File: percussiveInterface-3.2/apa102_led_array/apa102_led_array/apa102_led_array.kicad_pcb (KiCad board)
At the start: 2 copper layers, 167 x 10.2 mm, 49 parts

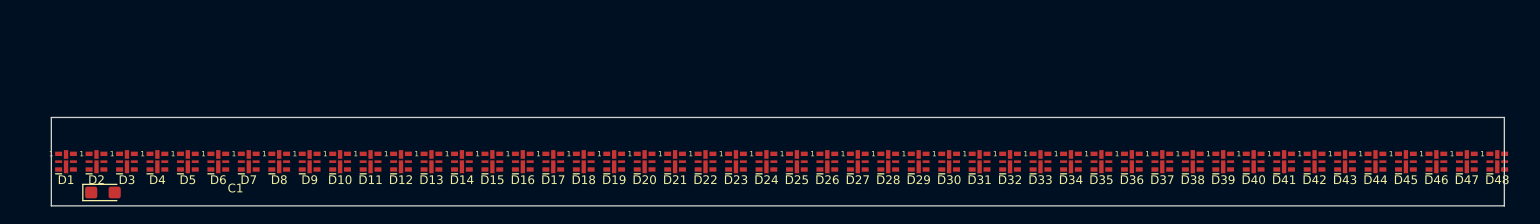
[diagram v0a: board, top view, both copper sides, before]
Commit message: many changes
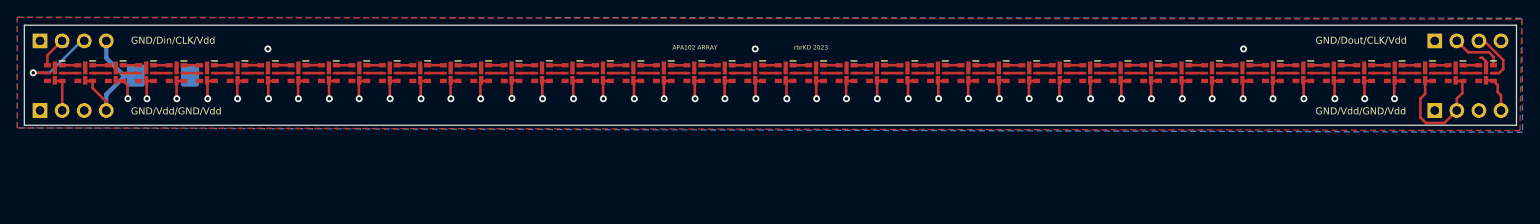
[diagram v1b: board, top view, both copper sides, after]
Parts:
- added REF**: PinHeader_1x04_P2.54mm_Vertical, Connector_PinHeader_2.54mm:PinHeader_1x04_P2.54mm_Vertical, B.Cu at (36.8, 29.3)
- added REF**: PinHeader_1x04_P2.54mm_Vertical, Connector_PinHeader_2.54mm:PinHeader_1x04_P2.54mm_Vertical, B.Cu at (197.1, 37.3)
- added REF**: PinHeader_1x04_P2.54mm_Vertical, Connector_PinHeader_2.54mm:PinHeader_1x04_P2.54mm_Vertical, B.Cu at (197.1, 29.3)
- added REF**: PinHeader_1x04_P2.54mm_Vertical, Connector_PinHeader_2.54mm:PinHeader_1x04_P2.54mm_Vertical, B.Cu at (36.8, 37.3)
- C1: footprint Capacitor_Tantalum_SMD:CP_EIA-3216-18_Kemet-A -> Capacitor_Tantalum_SMD:CP_EIA-7343-15_Kemet-W; moved to B.Cu
- moved C1 15.1 mm to (50.9, 33.3)
- moved D10 10.3 mm to (70.0, 33.0), turned to 180 degrees
- moved D11 10.3 mm to (73.5, 33.0), turned to 180 degrees
- moved D12 10.3 mm to (77.0, 33.0), turned to 180 degrees
- moved D13 10.3 mm to (80.5, 33.0), turned to 180 degrees
- moved D14 10.3 mm to (84.0, 33.0), turned to 180 degrees
- moved D15 10.3 mm to (87.5, 33.0), turned to 180 degrees
- moved D16 10.3 mm to (91.0, 33.0), turned to 180 degrees
- moved D17 10.3 mm to (94.5, 33.0), turned to 180 degrees
- moved D18 10.3 mm to (98.0, 33.0), turned to 180 degrees
- moved D19 10.3 mm to (101.5, 33.0), turned to 180 degrees
- moved D20 10.3 mm to (105.0, 33.0), turned to 180 degrees
- moved D21 10.3 mm to (108.5, 33.0), turned to 180 degrees
- moved D22 10.3 mm to (112.0, 33.0), turned to 180 degrees
- moved D23 10.3 mm to (115.5, 33.0), turned to 180 degrees
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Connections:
- D10 pad 2: Net-(D1-CKO) -> Net-(D10-CKO)
- D10 pad 3: Net-(D1-SDO) -> Net-(D10-SDO)
- D10 pad 4: DATA_IN -> Net-(D10-SDI)
- D10 pad 5: CLK_IN -> Net-(D10-CKI)
- D11 pad 2: Net-(D1-CKO) -> Net-(D11-CKO)
- D11 pad 3: Net-(D1-SDO) -> Net-(D11-SDO)
- D11 pad 4: DATA_IN -> Net-(D10-SDO)
- D11 pad 5: CLK_IN -> Net-(D10-CKO)
- D12 pad 2: Net-(D1-CKO) -> Net-(D12-CKO)
- D12 pad 3: Net-(D1-SDO) -> Net-(D12-SDO)
- D12 pad 4: DATA_IN -> Net-(D11-SDO)
- D12 pad 5: CLK_IN -> Net-(D11-CKO)
- D13 pad 2: Net-(D1-CKO) -> Net-(D13-CKO)
- D13 pad 3: Net-(D1-SDO) -> Net-(D13-SDO)
- D13 pad 4: DATA_IN -> Net-(D12-SDO)
- D13 pad 5: CLK_IN -> Net-(D12-CKO)
- D14 pad 2: Net-(D1-CKO) -> Net-(D14-CKO)
- D14 pad 3: Net-(D1-SDO) -> Net-(D14-SDO)
- D14 pad 4: DATA_IN -> Net-(D13-SDO)
- D14 pad 5: CLK_IN -> Net-(D13-CKO)
- D15 pad 2: Net-(D1-CKO) -> Net-(D15-CKO)
- D15 pad 3: Net-(D1-SDO) -> Net-(D15-SDO)
- D15 pad 4: DATA_IN -> Net-(D14-SDO)
- D15 pad 5: CLK_IN -> Net-(D14-CKO)
- D16 pad 2: Net-(D1-CKO) -> Net-(D16-CKO)
- D16 pad 3: Net-(D1-SDO) -> Net-(D16-SDO)
- D16 pad 4: DATA_IN -> Net-(D15-SDO)
- D16 pad 5: CLK_IN -> Net-(D15-CKO)
- D17 pad 2: Net-(D1-CKO) -> Net-(D17-CKO)
- D17 pad 3: Net-(D1-SDO) -> Net-(D17-SDO)
- D17 pad 4: DATA_IN -> Net-(D16-SDO)
- D17 pad 5: CLK_IN -> Net-(D16-CKO)
- D18 pad 2: Net-(D1-CKO) -> Net-(D18-CKO)
- D18 pad 3: Net-(D1-SDO) -> Net-(D18-SDO)
- D18 pad 4: DATA_IN -> Net-(D17-SDO)
- D18 pad 5: CLK_IN -> Net-(D17-CKO)
- D19 pad 2: Net-(D1-CKO) -> Net-(D19-CKO)
- D19 pad 3: Net-(D1-SDO) -> Net-(D19-SDO)
- D19 pad 4: DATA_IN -> Net-(D18-SDO)
- D19 pad 5: CLK_IN -> Net-(D18-CKO)
- D2 pad 2: Net-(D1-CKO) -> Net-(D2-CKO)
- D2 pad 3: Net-(D1-SDO) -> Net-(D2-SDO)
- D2 pad 4: DATA_IN -> Net-(D1-SDO)
- D2 pad 5: CLK_IN -> Net-(D1-CKO)
- D20 pad 2: Net-(D1-CKO) -> Net-(D20-CKO)
- D20 pad 3: Net-(D1-SDO) -> Net-(D20-SDO)
- D20 pad 4: DATA_IN -> Net-(D19-SDO)
- D20 pad 5: CLK_IN -> Net-(D19-CKO)
- D21 pad 2: Net-(D1-CKO) -> Net-(D21-CKO)
- D21 pad 3: Net-(D1-SDO) -> Net-(D21-SDO)
- D21 pad 4: DATA_IN -> Net-(D20-SDO)
- D21 pad 5: CLK_IN -> Net-(D20-CKO)
- D22 pad 2: Net-(D1-CKO) -> Net-(D22-CKO)
- D22 pad 3: Net-(D1-SDO) -> Net-(D22-SDO)
- D22 pad 4: DATA_IN -> Net-(D21-SDO)
- D22 pad 5: CLK_IN -> Net-(D21-CKO)
- D23 pad 2: Net-(D1-CKO) -> Net-(D23-CKO)
- D23 pad 3: Net-(D1-SDO) -> Net-(D23-SDO)
- D23 pad 4: DATA_IN -> Net-(D22-SDO)
- D23 pad 5: CLK_IN -> Net-(D22-CKO)
- D24 pad 2: Net-(D1-CKO) -> Net-(D24-CKO)
- D24 pad 3: Net-(D1-SDO) -> Net-(D24-SDO)
- D24 pad 4: DATA_IN -> Net-(D23-SDO)
- D24 pad 5: CLK_IN -> Net-(D23-CKO)
- D25 pad 2: Net-(D1-CKO) -> Net-(D25-CKO)
- D25 pad 3: Net-(D1-SDO) -> Net-(D25-SDO)
- D25 pad 4: DATA_IN -> Net-(D24-SDO)
- D25 pad 5: CLK_IN -> Net-(D24-CKO)
- D26 pad 2: Net-(D1-CKO) -> Net-(D26-CKO)
- D26 pad 3: Net-(D1-SDO) -> Net-(D26-SDO)
- D26 pad 4: DATA_IN -> Net-(D25-SDO)
- D26 pad 5: CLK_IN -> Net-(D25-CKO)
- D27 pad 2: Net-(D1-CKO) -> Net-(D27-CKO)
- D27 pad 3: Net-(D1-SDO) -> Net-(D27-SDO)
- D27 pad 4: DATA_IN -> Net-(D26-SDO)
- D27 pad 5: CLK_IN -> Net-(D26-CKO)
- D28 pad 2: Net-(D1-CKO) -> Net-(D28-CKO)
- D28 pad 3: Net-(D1-SDO) -> Net-(D28-SDO)
- D28 pad 4: DATA_IN -> Net-(D27-SDO)
- D28 pad 5: CLK_IN -> Net-(D27-CKO)
- D29 pad 2: Net-(D1-CKO) -> Net-(D29-CKO)
- D29 pad 3: Net-(D1-SDO) -> Net-(D29-SDO)
- D29 pad 4: DATA_IN -> Net-(D28-SDO)
- D29 pad 5: CLK_IN -> Net-(D28-CKO)
- D3 pad 2: Net-(D1-CKO) -> Net-(D3-CKO)
- D3 pad 3: Net-(D1-SDO) -> Net-(D3-SDO)
- D3 pad 4: DATA_IN -> Net-(D2-SDO)
- D3 pad 5: CLK_IN -> Net-(D2-CKO)
- D30 pad 2: Net-(D1-CKO) -> Net-(D30-CKO)
- D30 pad 3: Net-(D1-SDO) -> Net-(D30-SDO)
- D30 pad 4: DATA_IN -> Net-(D29-SDO)
- D30 pad 5: CLK_IN -> Net-(D29-CKO)
- D31 pad 2: Net-(D1-CKO) -> Net-(D31-CKO)
- D31 pad 3: Net-(D1-SDO) -> Net-(D31-SDO)
- D31 pad 4: DATA_IN -> Net-(D30-SDO)
- D31 pad 5: CLK_IN -> Net-(D30-CKO)
- D32 pad 2: Net-(D1-CKO) -> Net-(D32-CKO)
- D32 pad 3: Net-(D1-SDO) -> Net-(D32-SDO)
- D32 pad 4: DATA_IN -> Net-(D31-SDO)
- D32 pad 5: CLK_IN -> Net-(D31-CKO)
- D33 pad 2: Net-(D1-CKO) -> Net-(D33-CKO)
- D33 pad 3: Net-(D1-SDO) -> Net-(D33-SDO)
- D33 pad 4: DATA_IN -> Net-(D32-SDO)
- D33 pad 5: CLK_IN -> Net-(D32-CKO)
- D34 pad 2: Net-(D1-CKO) -> Net-(D34-CKO)
- D34 pad 3: Net-(D1-SDO) -> Net-(D34-SDO)
- D34 pad 4: DATA_IN -> Net-(D33-SDO)
- D34 pad 5: CLK_IN -> Net-(D33-CKO)
- D35 pad 2: Net-(D1-CKO) -> Net-(D35-CKO)
- D35 pad 3: Net-(D1-SDO) -> Net-(D35-SDO)
- D35 pad 4: DATA_IN -> Net-(D34-SDO)
- D35 pad 5: CLK_IN -> Net-(D34-CKO)
- D36 pad 2: Net-(D1-CKO) -> Net-(D36-CKO)
- D36 pad 3: Net-(D1-SDO) -> Net-(D36-SDO)
- D36 pad 4: DATA_IN -> Net-(D35-SDO)
- D36 pad 5: CLK_IN -> Net-(D35-CKO)
- D37 pad 2: Net-(D1-CKO) -> Net-(D37-CKO)
- D37 pad 3: Net-(D1-SDO) -> Net-(D37-SDO)
- D37 pad 4: DATA_IN -> Net-(D36-SDO)
- D37 pad 5: CLK_IN -> Net-(D36-CKO)
- D38 pad 2: Net-(D1-CKO) -> Net-(D38-CKO)
- D38 pad 3: Net-(D1-SDO) -> Net-(D38-SDO)
- D38 pad 4: DATA_IN -> Net-(D37-SDO)
- D38 pad 5: CLK_IN -> Net-(D37-CKO)
- D39 pad 2: Net-(D1-CKO) -> Net-(D39-CKO)
- D39 pad 3: Net-(D1-SDO) -> Net-(D39-SDO)
- D39 pad 4: DATA_IN -> Net-(D38-SDO)
- D39 pad 5: CLK_IN -> Net-(D38-CKO)
- D4 pad 2: Net-(D1-CKO) -> Net-(D4-CKO)
- D4 pad 3: Net-(D1-SDO) -> Net-(D4-SDO)
- D4 pad 4: DATA_IN -> Net-(D3-SDO)
- D4 pad 5: CLK_IN -> Net-(D3-CKO)
- D40 pad 2: Net-(D1-CKO) -> Net-(D40-CKO)
- D40 pad 3: Net-(D1-SDO) -> Net-(D40-SDO)
- D40 pad 4: DATA_IN -> Net-(D39-SDO)
- D40 pad 5: CLK_IN -> Net-(D39-CKO)
- D41 pad 2: Net-(D1-CKO) -> Net-(D41-CKO)
- D41 pad 3: Net-(D1-SDO) -> Net-(D41-SDO)
- D41 pad 4: DATA_IN -> Net-(D40-SDO)
- D41 pad 5: CLK_IN -> Net-(D40-CKO)
- D42 pad 2: Net-(D1-CKO) -> Net-(D42-CKO)
- D42 pad 3: Net-(D1-SDO) -> Net-(D42-SDO)
- D42 pad 4: DATA_IN -> Net-(D41-SDO)
- D42 pad 5: CLK_IN -> Net-(D41-CKO)
- D43 pad 2: Net-(D1-CKO) -> Net-(D43-CKO)
- D43 pad 3: Net-(D1-SDO) -> Net-(D43-SDO)
- D43 pad 4: DATA_IN -> Net-(D42-SDO)
- D43 pad 5: CLK_IN -> Net-(D42-CKO)
- D44 pad 2: Net-(D1-CKO) -> Net-(D44-CKO)
- D44 pad 3: Net-(D1-SDO) -> Net-(D44-SDO)
- D44 pad 4: DATA_IN -> Net-(D43-SDO)
- D44 pad 5: CLK_IN -> Net-(D43-CKO)
- D45 pad 2: Net-(D1-CKO) -> Net-(D45-CKO)
- D45 pad 3: Net-(D1-SDO) -> Net-(D45-SDO)
- D45 pad 4: DATA_IN -> Net-(D44-SDO)
- D45 pad 5: CLK_IN -> Net-(D44-CKO)
- D46 pad 2: Net-(D1-CKO) -> Net-(D46-CKO)
- D46 pad 3: Net-(D1-SDO) -> Net-(D46-SDO)
- D46 pad 4: DATA_IN -> Net-(D45-SDO)
- D46 pad 5: CLK_IN -> Net-(D45-CKO)
- D47 pad 2: Net-(D1-CKO) -> Net-(D47-CKO)
- D47 pad 3: Net-(D1-SDO) -> Net-(D47-SDO)
- D47 pad 4: DATA_IN -> Net-(D46-SDO)
- D47 pad 5: CLK_IN -> Net-(D46-CKO)
- D48 pad 2: Net-(D1-CKO) -> CLK_IN
- D48 pad 3: Net-(D1-SDO) -> DATA_IN
- D48 pad 4: DATA_IN -> Net-(D47-SDO)
- D48 pad 5: CLK_IN -> Net-(D47-CKO)
- D5 pad 2: Net-(D1-CKO) -> Net-(D5-CKO)
- D5 pad 3: Net-(D1-SDO) -> Net-(D5-SDO)
- D5 pad 4: DATA_IN -> Net-(D4-SDO)
- D5 pad 5: CLK_IN -> Net-(D4-CKO)
- D6 pad 2: Net-(D1-CKO) -> Net-(D6-CKO)
- D6 pad 3: Net-(D1-SDO) -> Net-(D6-SDO)
- D6 pad 4: DATA_IN -> Net-(D5-SDO)
- D6 pad 5: CLK_IN -> Net-(D5-CKO)
- D7 pad 2: Net-(D1-CKO) -> Net-(D7-CKO)
- D7 pad 3: Net-(D1-SDO) -> Net-(D7-SDO)
- D7 pad 4: DATA_IN -> Net-(D6-SDO)
- D7 pad 5: CLK_IN -> Net-(D6-CKO)
- D8 pad 2: Net-(D1-CKO) -> Net-(D8-CKO)
- D8 pad 3: Net-(D1-SDO) -> Net-(D8-SDO)
- D8 pad 4: DATA_IN -> Net-(D7-SDO)
- D8 pad 5: CLK_IN -> Net-(D7-CKO)
- D9 pad 2: Net-(D1-CKO) -> Net-(D10-CKI)
- D9 pad 3: Net-(D1-SDO) -> Net-(D10-SDI)
- D9 pad 4: DATA_IN -> Net-(D8-SDO)
- D9 pad 5: CLK_IN -> Net-(D8-CKO)
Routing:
- net Vdd: track 0.00 -> 164.0 mm, vias 0 -> 43
- net CLK_IN: track 0.00 -> 15.1 mm, vias 0 -> 1
- net DATA_IN: track 0.00 -> 10.1 mm
- net Net-(D47-SDO): track 0.00 -> 1.80 mm
- net Net-(D47-CKO): track 0.00 -> 1.80 mm
- net Net-(D46-SDO): track 0.00 -> 1.80 mm
- net Net-(D46-CKO): track 0.00 -> 1.80 mm
- net Net-(D45-SDO): track 0.00 -> 1.80 mm
- net Net-(D45-CKO): track 0.00 -> 1.80 mm
- net Net-(D44-SDO): track 0.00 -> 1.80 mm
- net Net-(D44-CKO): track 0.00 -> 1.80 mm
- net Net-(D43-SDO): track 0.00 -> 1.80 mm
- net Net-(D43-CKO): track 0.00 -> 1.80 mm
- net Net-(D42-SDO): track 0.00 -> 1.80 mm
- net Net-(D42-CKO): track 0.00 -> 1.80 mm
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- added copper zone on B.Cu, net GND
- added copper zone on F.Cu, net GND
- added copper zone on In2.Cu, net GND
- added copper zone on In1.Cu, net Vdd
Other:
- board size 167 x 10.2 mm -> 171.5 x 11.5 mm
- copper layers 2 -> 4
- board text added: "APA102 ARRAY"
- board text added: "GND/Din/CLK/Vdd"
- board text added: "GND/Dout/CLK/Vdd"
- board text added: "GND/Vdd/GND/Vdd"
- board text added: "rbrKD 2023"

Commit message: quadrillion changes
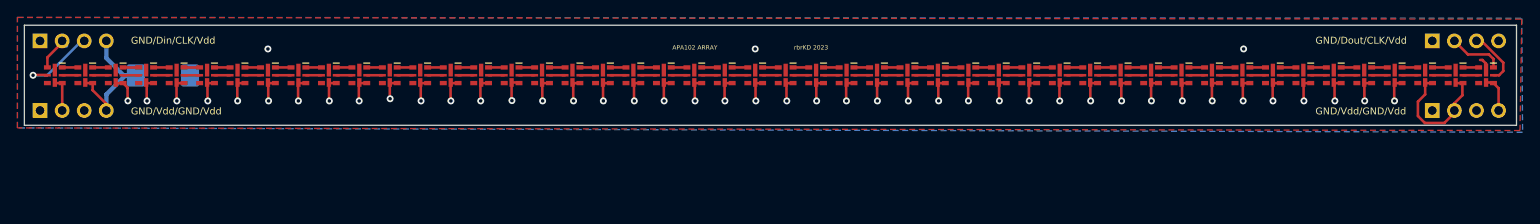
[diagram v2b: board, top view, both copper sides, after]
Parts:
- moved REF** 0.28 mm to (196.8, 37.3)
- moved REF** 0.28 mm to (196.8, 29.3)
- moved D1 0.25 mm to (38.5, 33.2)
- moved D10 0.25 mm to (70.0, 33.2)
- moved D11 0.25 mm to (73.5, 33.2)
- moved D12 0.25 mm to (77.0, 33.2)
- moved D13 0.25 mm to (80.5, 33.2)
- moved D14 0.25 mm to (84.0, 33.2)
- moved D15 0.25 mm to (87.5, 33.2)
- moved D16 0.25 mm to (91.0, 33.2)
- moved D17 0.25 mm to (94.5, 33.2)
- moved D18 0.25 mm to (98.0, 33.2)
- moved D19 0.25 mm to (101.5, 33.2)
- moved D2 0.25 mm to (42.0, 33.2)
- moved D20 0.25 mm to (105.0, 33.2)
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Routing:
- net CLK_IN: track 15.1 -> 15.8 mm
